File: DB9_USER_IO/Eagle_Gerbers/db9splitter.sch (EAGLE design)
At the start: 19 parts, among them IC1 74LVC1G04DBV

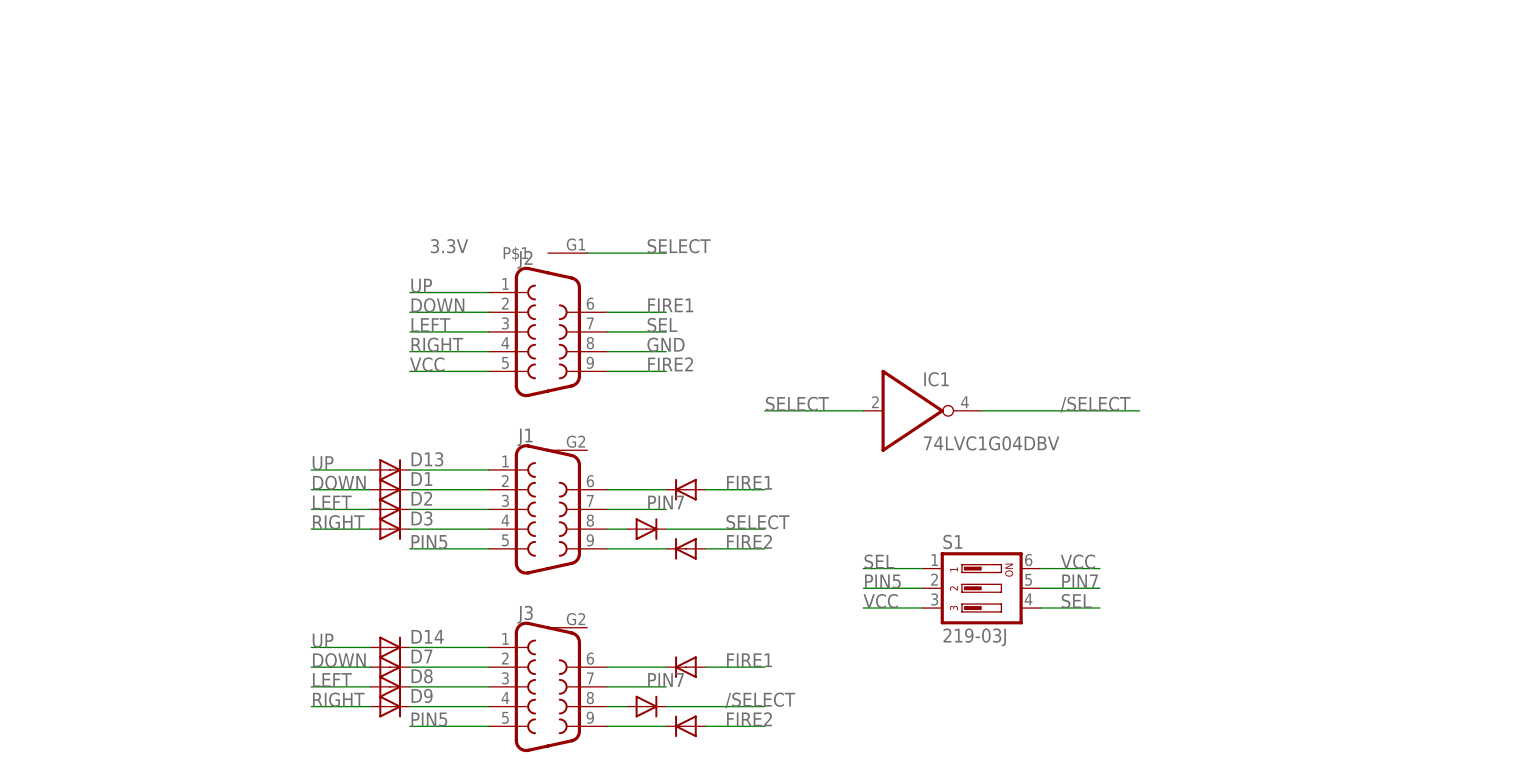
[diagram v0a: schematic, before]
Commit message: updated db9splitter
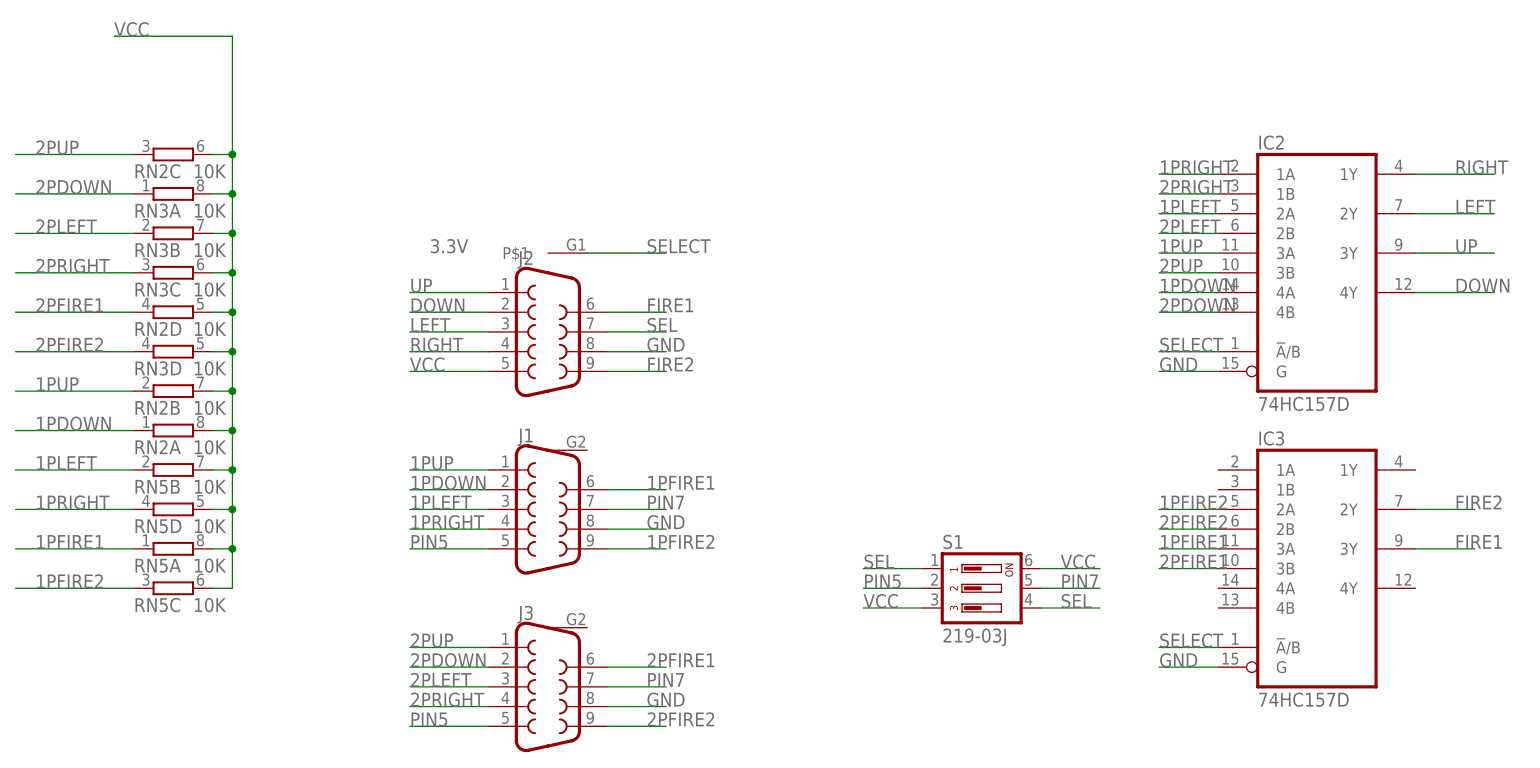
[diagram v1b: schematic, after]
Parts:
- removed D1, D10, D11, D12, D13, D14, D2, D3, D4, D5, D6, D7, D8, D9: (no value), diode:DIODE-SOD323-R
- removed IC1: 74LVC1G04DBV, 74xx-little-de:74LVC1G04DBV
- added IC2, IC3: 74HC157D, 74xx-eu:74HC157D
- added RN2, RN3, RN5: 10K, resistor-dil:4R-N0603-ARC
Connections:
- removed net /SELECT: D10.C, IC1A.O
- removed net N$1: D13.C, J1.1
- removed net N$11: D6.C, J1.9
- removed net N$12: D5.C, J1.6
- removed net N$13: D12.C, J3.9
- removed net N$14: D11.C, J3.6
- removed net N$15: D4.A, J1.8
- removed net N$2: D14.C, J3.1
- removed net N$3: D2.C, J1.3
- removed net N$4: D8.C, J3.3
- removed net N$5: D1.C, J1.2
- removed net N$6: D3.C, J1.4
- removed net N$7: D7.C, J3.2
- removed net N$8: D9.C, J3.4
- removed net N$9: D10.A, J3.8
- new net 1PDOWN: IC2A.4A, J1.2, RN2A.1
- new net 1PFIRE1: IC3A.3A, J1.6, RN5A.1
- new net 1PFIRE2: IC3A.2A, J1.9, RN5C.1
- new net 1PLEFT: IC2A.2A, J1.3, RN5B.1
- new net 1PRIGHT: IC2A.1A, J1.4, RN5D.1
- new net 1PUP: IC2A.3A, J1.1, RN2B.1
- new net 2PDOWN: IC2A.4B, J3.2, RN3A.1
- new net 2PFIRE1: IC3A.3B, J3.6, RN2D.1
- new net 2PFIRE2: IC3A.2B, J3.9, RN3D.1
- new net 2PLEFT: IC2A.2B, J3.3, RN3B.1
- new net 2PRIGHT: IC2A.1B, J3.4, RN3C.1
- new net 2PUP: IC2A.3B, J3.1, RN2C.1
- net DOWN: now also IC2A.4Y; no longer D1.A, D7.A
- net FIRE1: now also IC3A.3Y; no longer D11.A, D5.A
- net FIRE2: now also IC3A.2Y; no longer D12.A, D6.A
- net GND: now also IC2A.G, IC3A.G, J1.8, J3.8
- net LEFT: now also IC2A.2Y; no longer D2.A, D8.A
- net RIGHT: now also IC2A.1Y; no longer D3.A, D9.A
- net SELECT: now also IC2A.!A!/B, IC3A.!A!/B; no longer D4.C, IC1A.I
- net UP: now also IC2A.3Y; no longer D13.A, D14.A
- net VCC: now also RN2A.2, RN2B.2, RN2C.2, RN2D.2, RN3A.2, RN3B.2, RN3C.2, RN3D.2, RN5A.2, RN5B.2, RN5C.2, RN5D.2
